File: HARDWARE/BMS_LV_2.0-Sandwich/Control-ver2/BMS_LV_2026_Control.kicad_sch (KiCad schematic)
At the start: 5 parts, among them J1 Conn_01x26

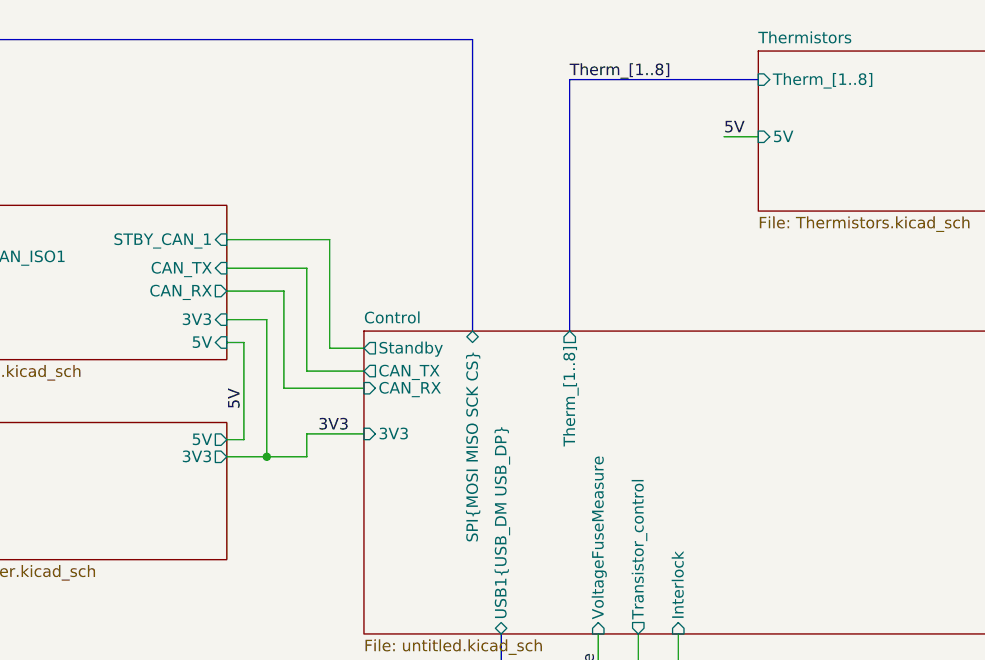
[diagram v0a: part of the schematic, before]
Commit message: Kolejna kurwa wersja gotowa, japierdole
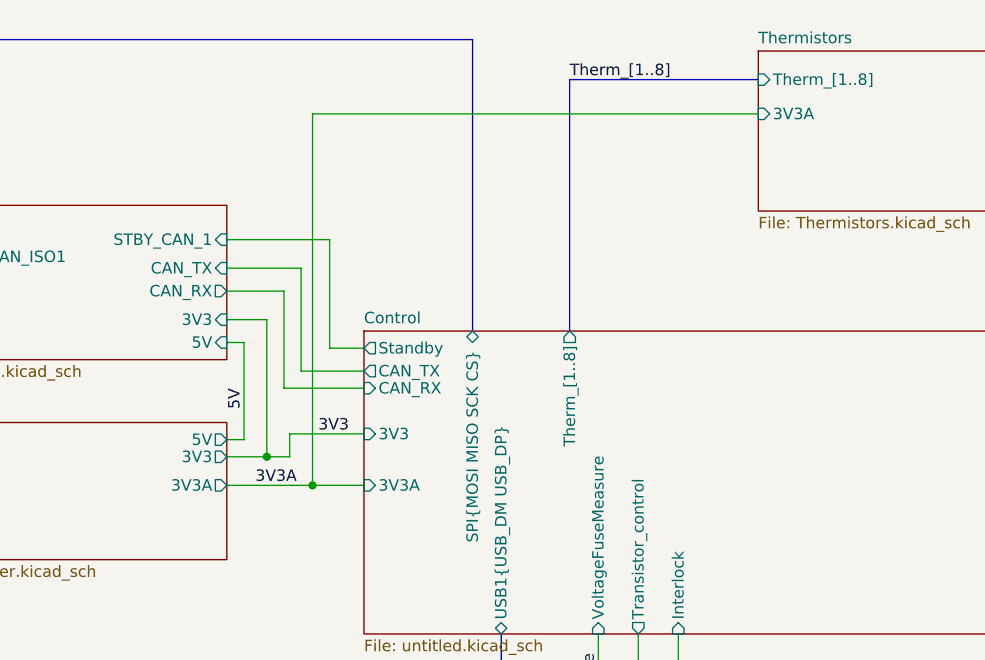
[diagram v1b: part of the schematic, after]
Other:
- sheet Control ports: added 3V3A; removed none
- sheet Power ports: added 3V3A; removed none
- sheet Thermistors ports: added 3V3A; removed 5V
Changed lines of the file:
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@@
+		(color 0 0 0 0)
+	)
+	(junction
+		(at 127.635 100.965)
+		(diameter 0)
 		(color 0 0 0 0)
 	)
@@
 	(wire
 		(pts
-			(xy 127 76.835) (xy 118.11 76.835)
+			(xy 126.365 76.835) (xy 118.11 76.835)
 		)
 		(stroke
@@
 	(wire
 		(pts
-			(xy 127 88.265) (xy 127 76.835)
+			(xy 126.365 88.265) (xy 126.365 76.835)
 		)
 		(stroke
@@
 	(wire
 		(pts
-			(xy 127 95.25) (xy 133.35 95.25)
+			(xy 125.095 95.25) (xy 133.35 95.25)
 		)
 		(stroke
@@
 	(wire
 		(pts
-			(xy 122.555 97.79) (xy 127 97.79)
+			(xy 122.555 97.79) (xy 125.095 97.79)
 		)
 		(stroke
@@
 	(wire
 		(pts
+			(xy 127.635 100.965) (xy 133.35 100.965)
+		)
+		(stroke
+			(width 0)
+			(type default)
+		)
+	)
+	(wire
+		(pts
 			(xy 57.15 95.885) (xy 34.29 95.885)
 		)
@@
 	(wire
 		(pts
+			(xy 177.165 59.69) (xy 127.635 59.69)
+		)
+		(stroke
+			(width 0)
+			(type default)
+		)
+	)
+	(wire
+		(pts
 			(xy 37.465 126.365) (xy 37.465 123.825)
 		)
@@
 	(wire
 		(pts
+			(xy 118.11 100.965) (xy 127.635 100.965)
+		)
+		(stroke
+			(width 0)
+			(type default)
+		)
+	)
+	(wire
+		(pts
 			(xy 129.54 73.66) (xy 118.11 73.66)
 		)
@@
 	(wire
 		(pts
-			(xy 133.35 88.265) (xy 127 88.265)
+			(xy 133.35 88.265) (xy 126.365 88.265)
 		)
 		(stroke
@@
 	(wire
 		(pts
+			(xy 127.635 59.69) (xy 127.635 100.965)
+		)
+		(stroke
+			(width 0)
+			(type default)
+		)
+	)
+	(wire
+		(pts
 			(xy 37.465 126.365) (xy 37.465 128.905)
 		)
@@
 	(wire
 		(pts
-			(xy 127 97.79) (xy 127 95.25)
+			(xy 125.095 97.79) (xy 125.095 95.25)
 		)
 		(stroke
@@
 		(pts
 			(xy 129.54 85.725) (xy 129.54 73.66)
-		)
-		(stroke
-			(width 0)
-			(type default)
-		)
-	)
-	(wire
-		(pts
-			(xy 173.355 62.23) (xy 177.165 62.23)
 		)
 		(stroke
@@
 		)
 	)
-	(label "5V"
-		(at 173.355 62.23 0)
-		(effects
-			(font
-				(size 1.27 1.27)
-			)
-			(justify left bottom)
-		)
-	)
 	(label "3V3"
 		(at 42.545 118.745 180)
@@
 	(label "CAN-"
 		(at 76.2 82.55 0)
+		(effects
+			(font
+				(size 1.27 1.27)
+			)
+			(justify left bottom)
+		)
+	)
+	(label "3V3A"
+		(at 121.285 100.965 0)
 		(effects
 			(font
@@
 			)
 		)
-		(pin "5V" input
-			(at 177.165 62.23 180)
+		(pin "3V3A" input
+			(at 177.165 59.69 180)
 			(effects
 				(font
@@
 			)
 		)
+		(pin "3V3A" output
+			(at 118.11 100.965 0)
+			(effects
+				(font
+					(size 1.27 1.27)
+				)
+				(justify right)
+			)
+		)
 		(instances
 			(project "BMS_LV_2026_Control"
@@
 			(effects
 				(font
+					(size 1.27 1.27)
+				)
+				(justify left)
+			)
+		)
+		(pin "3V3A" input
+			(at 133.35 100.965 180)
+			(effects
+				(font
